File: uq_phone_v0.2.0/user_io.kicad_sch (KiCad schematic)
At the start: 19 parts, among them J8 MCS-302S-C1, M1 C08-00A, U10 TPD8F003DQDR, U11 LSM6DSVTR, U12 DRV2603RUNR, U8 TPD3F303DQDR, U9 MCP1664T-E/OT

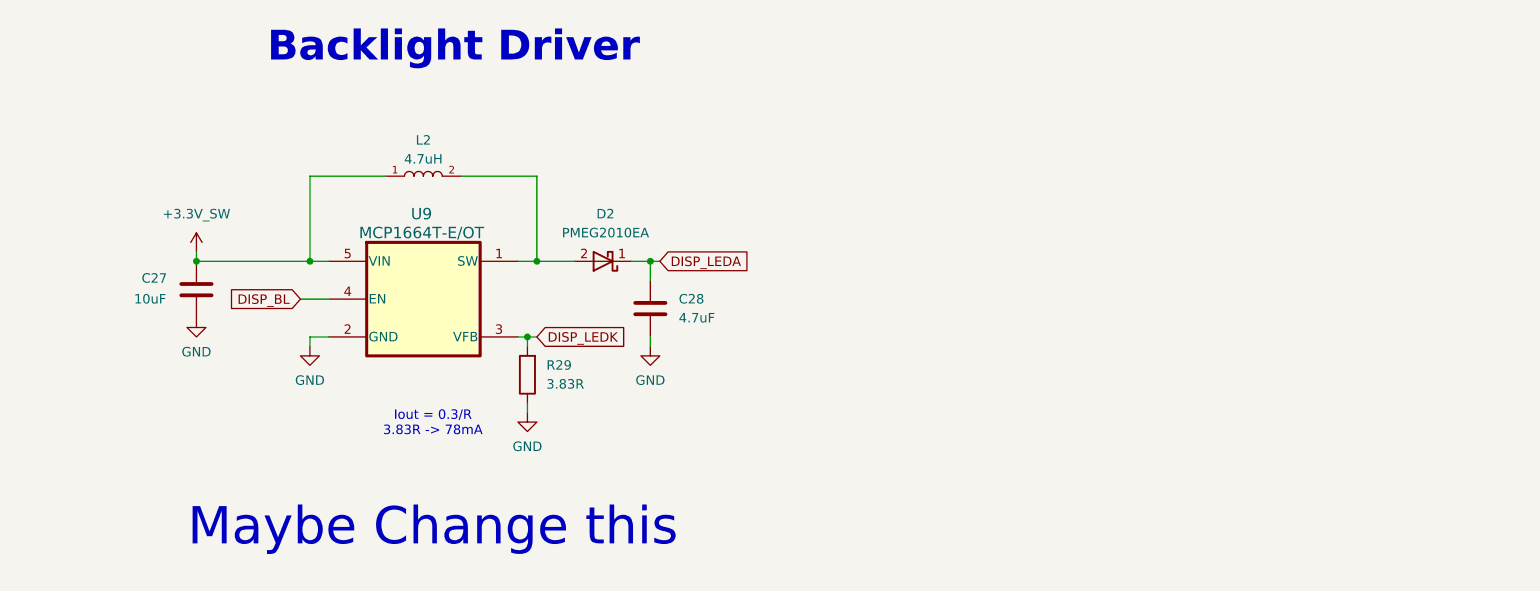
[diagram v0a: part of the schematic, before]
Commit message: New Layout
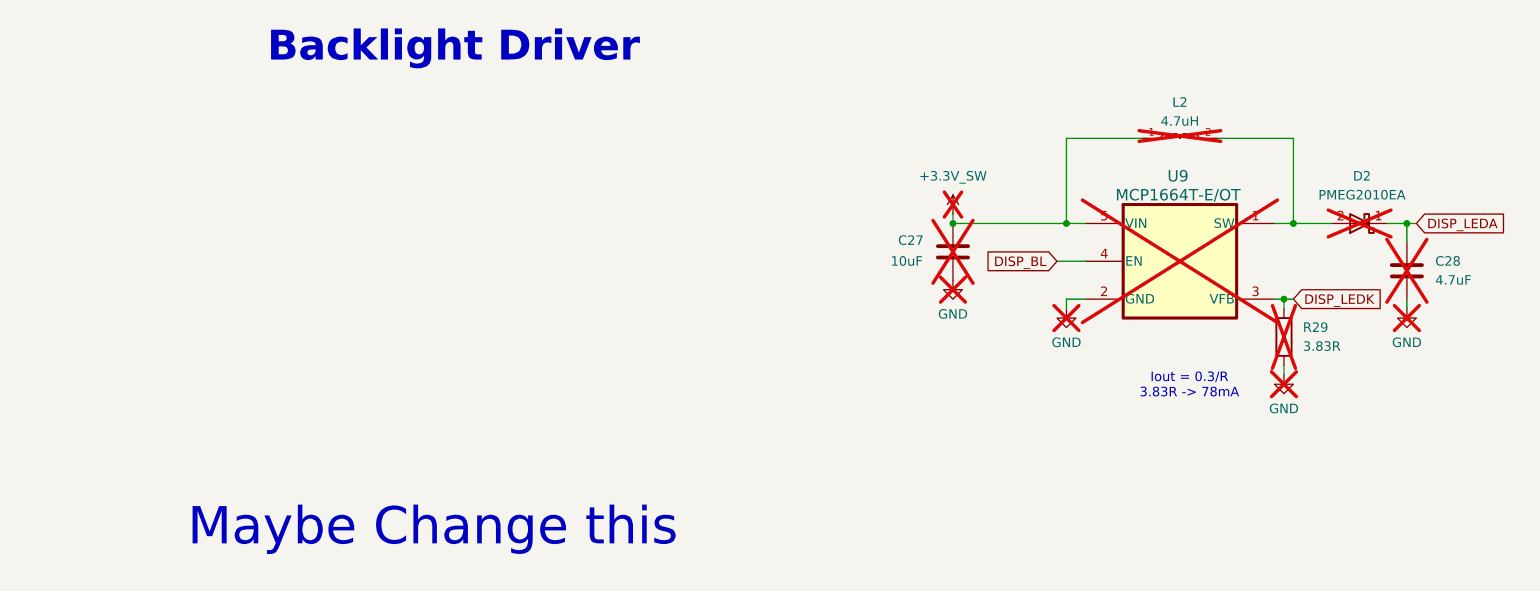
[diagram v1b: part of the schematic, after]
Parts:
- C27, C28, D2, L2, R29, U9: now not fitted
- DISP1: footprint (none) -> custom_footprints:Display
